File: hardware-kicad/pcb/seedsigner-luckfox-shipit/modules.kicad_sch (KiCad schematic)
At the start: 3 parts, among them U1 LuckFox_Pico_MINI, U2 LuckFox_Pico_PLUS_PRO

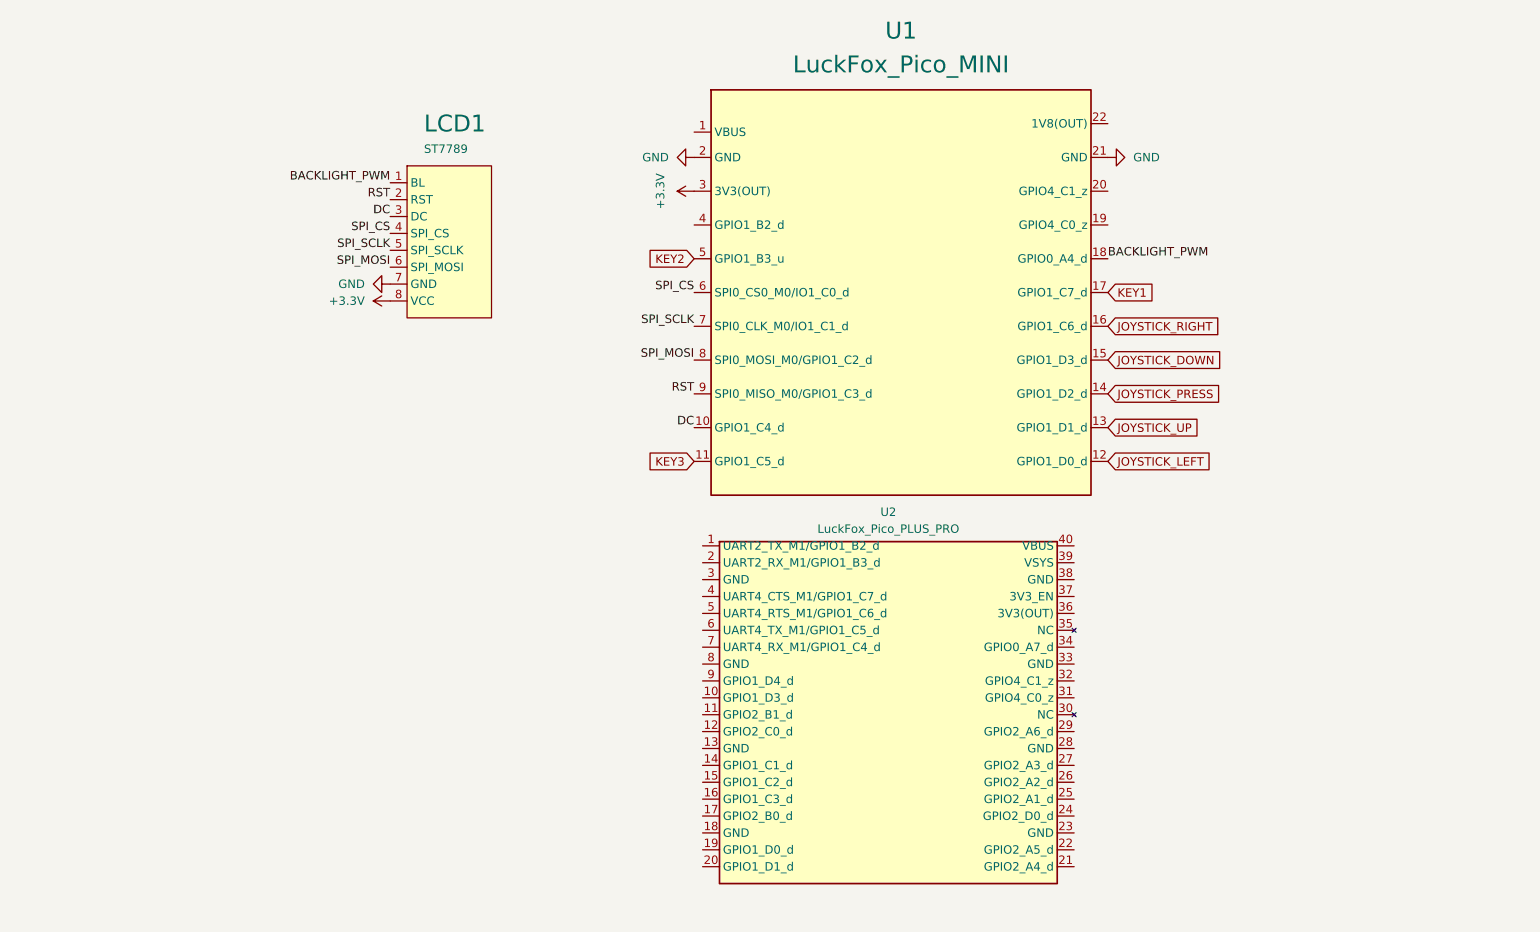
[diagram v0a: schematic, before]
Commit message: 2 different pcbs almost done
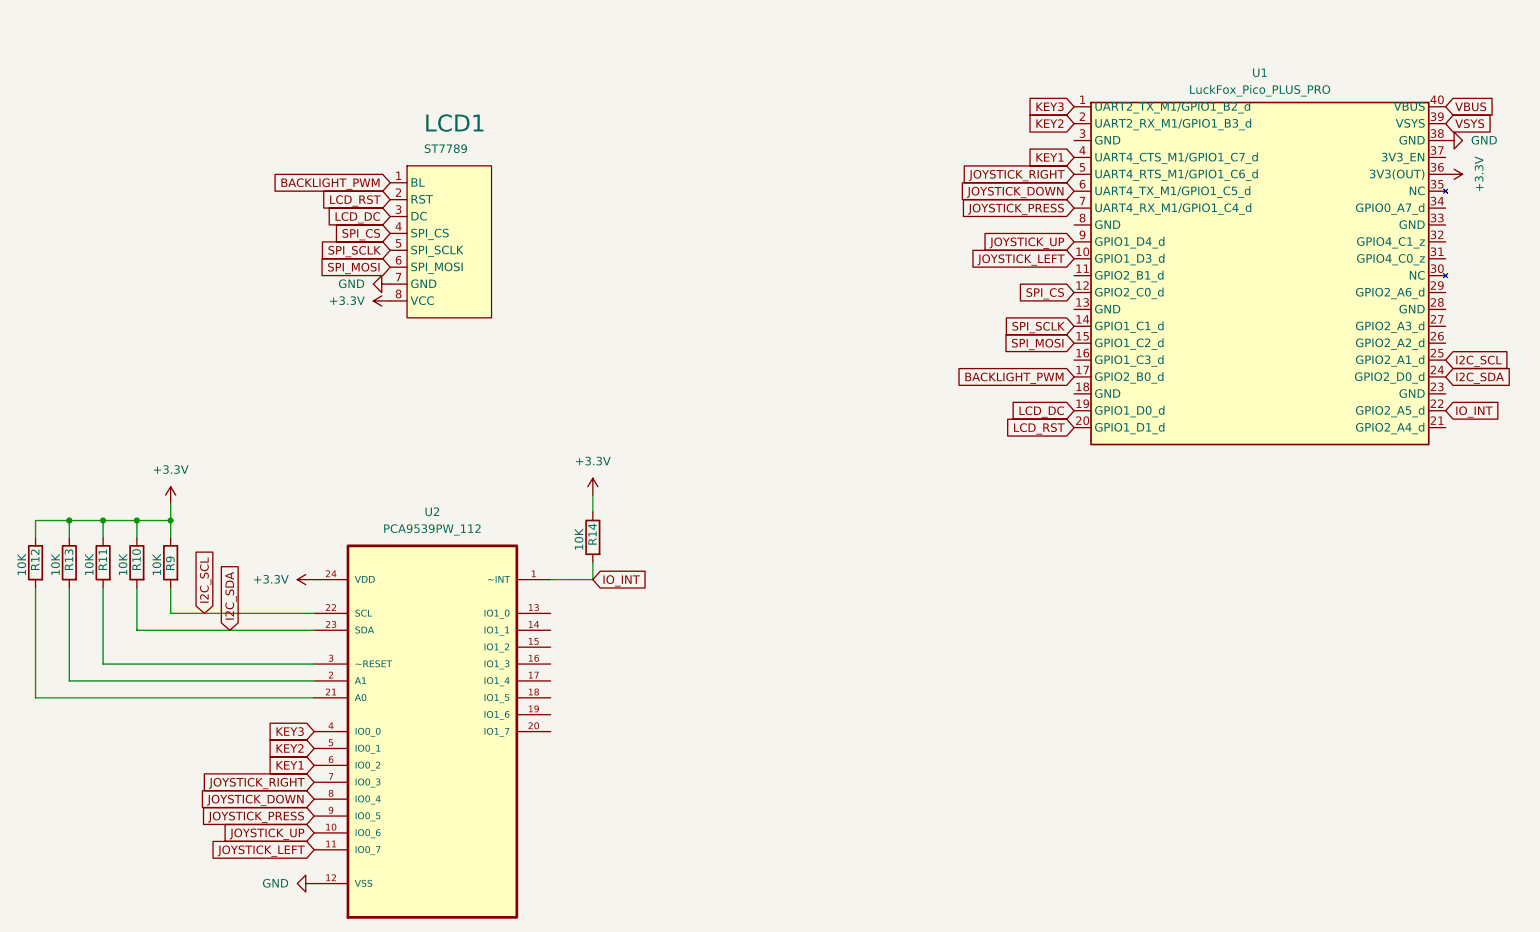
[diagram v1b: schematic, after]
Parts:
- removed U1: LuckFox_Pico_MINI, seedsigner-luckfox:LUCKFOX_PICO_MINI, symbol Luckfox:LuckFox_Pico_MINI
- added R10, R11, R12, R13, R14, R9: 10K, Resistor_SMD:R_0805_2012Metric_Pad1.20x1.40mm_HandSolder, symbol Device:R
- added U2: PCA9539PW_112, seedsigner-luckfox:SOP65P640X110-24N, symbol SeedSigner:PCA9539PW_112
- U1: renamed from U2; footprint (none) -> seedsigner-luckfox:LUCKFOX_PICO
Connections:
- net DC is gone; now on net LCD_DC: LCD1.3 (DC)
- net RST is gone; now on net LCD_RST: LCD1.2 (RST)
- net +3.3V: now also U1.36 (3V3(OUT)), R10.1, R11.1, R12.1, R13.1, R14.1, R9.1, U2.24 (VDD)
- net BACKLIGHT_PWM: now also U1.17 (GPIO2_B0_d)
- net GND: now also U1.38 (GND), U2.12 (VSS)
- net JOYSTICK_DOWN: now also U1.6 (UART4_TX_M1/GPIO1_C5_d), U2.8 (IO0_4)
- net JOYSTICK_LEFT: now also U1.10 (GPIO1_D3_d), U2.11 (IO0_7)
- net JOYSTICK_PRESS: now also U1.7 (UART4_RX_M1/GPIO1_C4_d), U2.9 (IO0_5)
- net JOYSTICK_RIGHT: now also U1.5 (UART4_RTS_M1/GPIO1_C6_d), U2.7 (IO0_3)
- net JOYSTICK_UP: now also U1.9 (GPIO1_D4_d), U2.10 (IO0_6)
- net KEY1: now also U1.4 (UART4_CTS_M1/GPIO1_C7_d), U2.6 (IO0_2)
- net KEY2: now also U1.2 (UART2_RX_M1/GPIO1_B3_d), U2.5 (IO0_1)
- net KEY3: now also U1.1 (UART2_TX_M1/GPIO1_B2_d), U2.4 (IO0_0)
- net SPI_CS: now also U1.12 (GPIO2_C0_d)
- net SPI_MOSI: now also U1.15 (GPIO1_C2_d)
- net SPI_SCLK: now also U1.14 (GPIO1_C1_d)
- net LCD_DC: now reaches U1.19 (GPIO1_D0_d)
- net LCD_RST: now reaches U1.20 (GPIO1_D1_d)
- net IO_INT: now reaches U1.22 (GPIO2_A5_d)
- net IO_INT: now also R14.2, U2.1 (~INT)
- net I2C_SDA: now reaches U1.24 (GPIO2_D0_d)
- net I2C_SDA: now also R10.2, U2.23 (SDA)
- net I2C_SCL: now reaches U1.25 (GPIO2_A1_d)
- net I2C_SCL: now also R9.2, U2.22 (SCL)
- net VSYS: now reaches U1.39 (VSYS)
- net VBUS: now reaches U1.40 (VBUS)
- new net: R13.2, U2.2 (A1)
- new net: R12.2, U2.21 (A0)
- new net: R11.2, U2.3 (~RESET)
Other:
- moved on the sheet: U1
